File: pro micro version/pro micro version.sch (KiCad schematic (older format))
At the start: 78 parts, among them SW1 SW_PUSH, U1 ProMicro

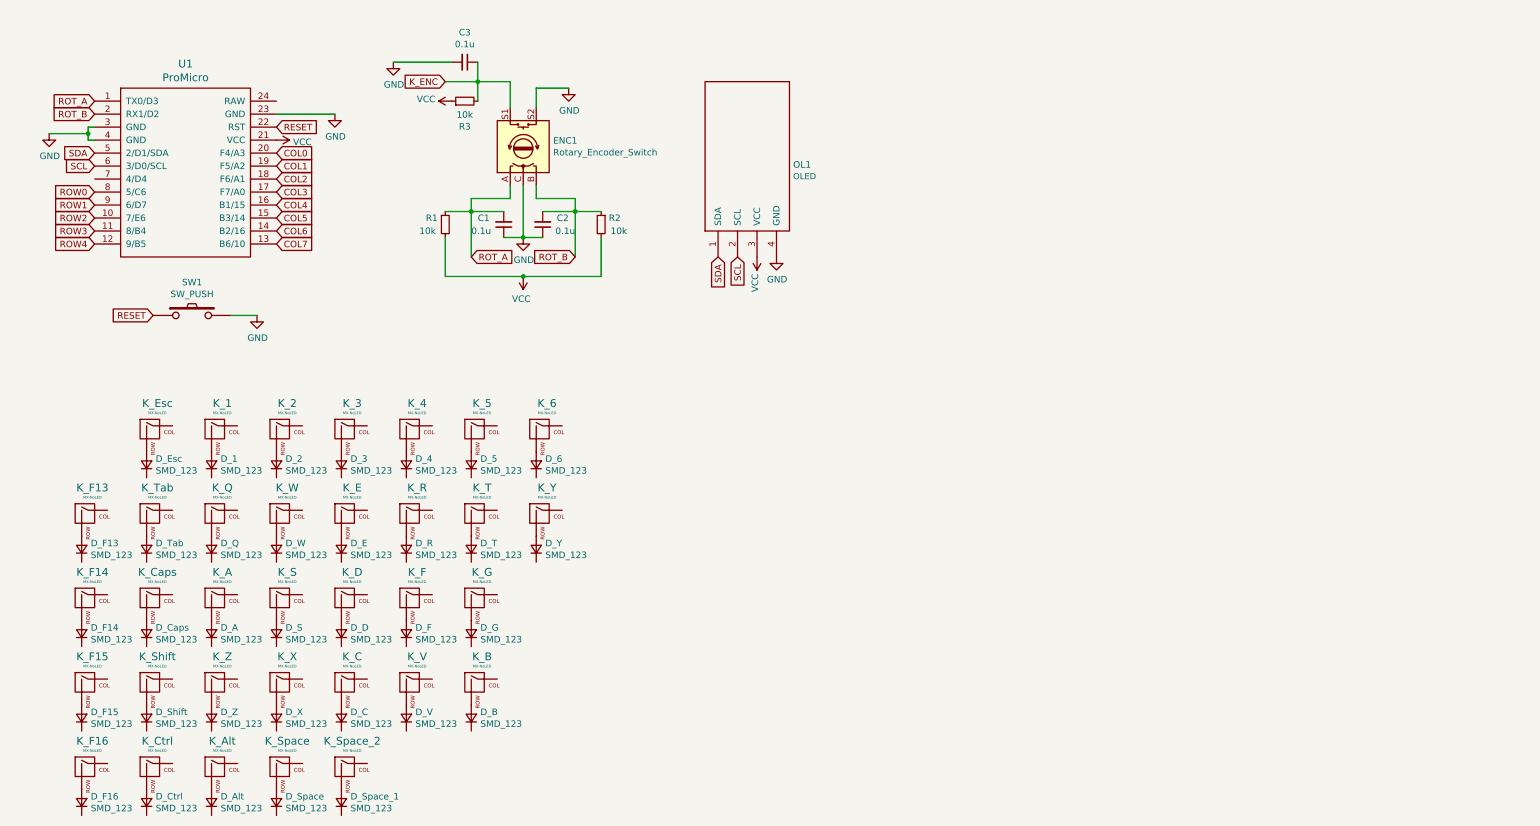
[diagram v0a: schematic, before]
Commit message: finished sechma
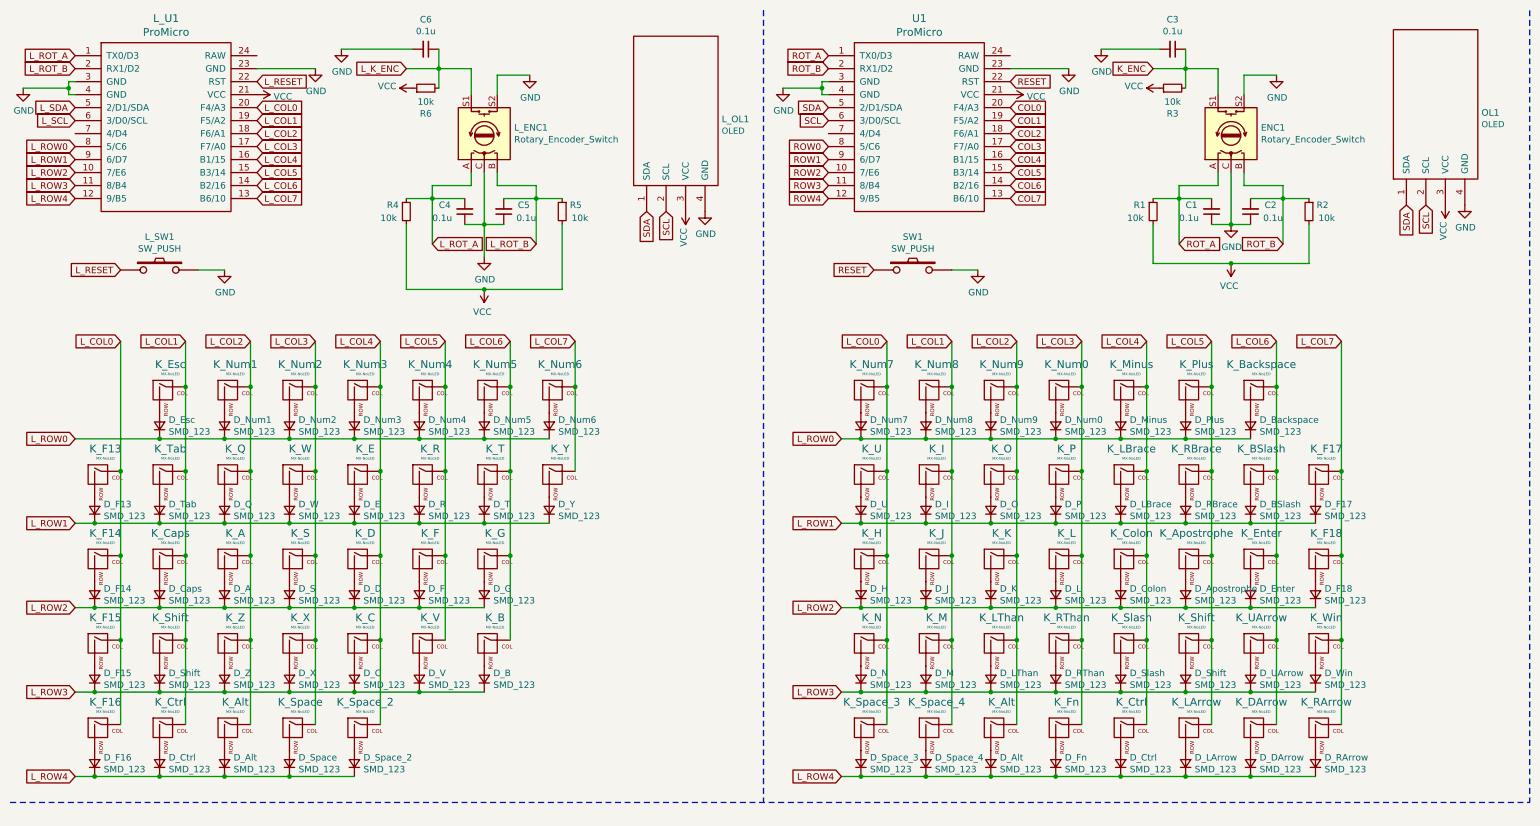
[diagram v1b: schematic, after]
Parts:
- added C1, C2, C3: 0.1u, symbol Device:C_Small
- added D_Alt, D_Apostrophe, D_BSlash, D_Backspace, D_Colon, D_Ctrl, D_DArrow, D_Enter, D_F17, D_F18, D_Fn, D_H, D_I, D_J, D_K, D_L, D_LArrow, D_LBrace, D_LThan, D_M, D_Minus, D_N, D_Num0, D_Num7, D_Num8, D_Num9, D_O, D_P, D_Plus, D_RArrow, D_RBrace, D_RThan, D_Shift, D_Slash, D_Space_3, D_Space_4, D_U, D_UArrow, D_Win: SMD_123, symbol Device:D_Small
- added ENC1: Rotary_Encoder_Switch, symbol Device:Rotary_Encoder_Switch
- added K_Alt, K_Apostrophe, K_BSlash, K_Backspace, K_Colon, K_Ctrl, K_DArrow, K_Enter, K_F17, K_F18, K_Fn, K_H, K_I, K_J, K_K, K_L, K_LArrow, K_LBrace, K_LThan, K_M, K_Minus, K_N, K_Num0, K_Num7, K_Num8, K_Num9, K_O, K_P, K_Plus, K_RArrow, K_RBrace, K_RThan, K_Shift, K_Slash, K_Space_3, K_Space_4, K_U, K_UArrow, K_Win: MX-NoLED, symbol MX_Alps_Hybrid:MX-NoLED
- added OL1: OLED, symbol kbd:OLED
- added R1, R2, R3: 10k, symbol Device:R_Small
- added SW1: SW_PUSH, symbol kbd:SW_PUSH
- added U1: ProMicro, symbol kbd:ProMicro
- renumbered C1 to C4, C2 to C5, C3 to C6, D_1 to D_Num1, D_2 to D_Num2, D_3 to D_Num3, D_4 to D_Num4, D_5 to D_Num5, D_6 to D_Num6, D_Space_1 to D_Space_2, K_1 to K_Num1, K_2 to K_Num2, K_3 to K_Num3, K_4 to K_Num4, K_5 to K_Num5, K_6 to K_Num6, ENC1 to L_ENC1, OL1 to L_OL1, SW1 to L_SW1, U1 to L_U1, R1 to R4, R2 to R5, R3 to R6
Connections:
- net COL0: now also U1.20 (F4/A3); no longer L_U1.20 (F4/A3)
- net COL1: now also U1.19 (F5/A2); no longer L_U1.19 (F5/A2)
- net COL2: now also U1.18 (F6/A1); no longer L_U1.18 (F6/A1)
- net COL3: now also U1.17 (F7/A0); no longer L_U1.17 (F7/A0)
- net COL4: now also U1.16 (B1/15); no longer L_U1.16 (B1/15)
- net COL5: now also U1.15 (B3/14); no longer L_U1.15 (B3/14)
- net COL6: now also U1.14 (B2/16); no longer L_U1.14 (B2/16)
- net COL7: now also U1.13 (B6/10); no longer L_U1.13 (B6/10)
- net GND: now also C1.1, C2.1, C3.2, ENC1.C, ENC1.S2, OL1.4 (GND), SW1.2, U1.23 (GND), U1.3 (GND), U1.4 (GND)
- net K_ENC: now also C3.1, ENC1.S1, R3.2; no longer C6.1, L_ENC1.S1, R6.2
- net RESET: now also SW1.1, U1.22 (RST); no longer L_SW1.1, L_U1.22 (RST)
- net ROT_A: now also C1.2, ENC1.A, R1.1, U1.1 (TX0/D3); no longer C4.2, L_ENC1.A, L_U1.1 (TX0/D3), R4.1
- net ROT_B: now also C2.2, ENC1.B, R2.1, U1.2 (RX1/D2); no longer C5.2, L_ENC1.B, L_U1.2 (RX1/D2), R5.1
- net ROW0: now also U1.8 (5/C6); no longer L_U1.8 (5/C6)
- net ROW1: now also U1.9 (6/D7); no longer L_U1.9 (6/D7)
- net ROW2: now also U1.10 (7/E6); no longer L_U1.10 (7/E6)
- net ROW3: now also U1.11 (8/B4); no longer L_U1.11 (8/B4)
- net ROW4: now also U1.12 (9/B5); no longer L_U1.12 (9/B5)
- net SCL: now also OL1.2 (SCL), U1.6 (3/D0/SCL); no longer L_U1.6 (3/D0/SCL)
- net SDA: now also OL1.1 (SDA), U1.5 (2/D1/SDA); no longer L_U1.5 (2/D1/SDA)
- net VCC: now also OL1.3 (VCC), R1.2, R2.2, R3.1, U1.21 (VCC)
- net L_COL1: now reaches K_Esc.1 (COL)
- net L_COL1: now also K_Caps.1 (COL), K_Ctrl.1 (COL), K_Shift.1 (COL), K_Tab.1 (COL), L_U1.19 (F5/A2), K_I.1 (COL), K_J.1 (COL), K_M.1 (COL), K_Num8.1 (COL), K_Space_4.1 (COL)
- net L_ROW0: now reaches D_Esc.1 (K)
- net L_ROW0: now also D_Num1.1 (K), D_Num2.1 (K), D_Num3.1 (K), D_Num4.1 (K), D_Num5.1 (K), D_Num6.1 (K), L_U1.8 (5/C6), D_Backspace.1 (K), D_Minus.1 (K), D_Num0.1 (K), D_Num7.1 (K), D_Num8.1 (K), D_Num9.1 (K), D_Plus.1 (K)
- net L_COL2: now reaches K_Num1.1 (COL)
- net L_COL2: now also K_A.1 (COL), K_Alt.1 (COL), K_Q.1 (COL), K_Z.1 (COL), L_U1.18 (F6/A1), K_Alt.1 (COL), K_K.1 (COL), K_LThan.1 (COL), K_Num9.1 (COL), K_O.1 (COL)
- net L_COL3: now reaches K_Num2.1 (COL)
- net L_COL3: now also K_S.1 (COL), K_Space.1 (COL), K_W.1 (COL), K_X.1 (COL), L_U1.17 (F7/A0), K_Fn.1 (COL), K_L.1 (COL), K_Num0.1 (COL), K_P.1 (COL), K_RThan.1 (COL)
- net L_COL4: now reaches K_Num3.1 (COL)
- net L_COL4: now also K_C.1 (COL), K_D.1 (COL), K_E.1 (COL), K_Space_2.1 (COL), L_U1.16 (B1/15), K_Colon.1 (COL), K_Ctrl.1 (COL), K_LBrace.1 (COL), K_Minus.1 (COL), K_Slash.1 (COL)
- net L_COL5: now reaches K_Num4.1 (COL)
- net L_COL5: now also K_F.1 (COL), K_R.1 (COL), K_V.1 (COL), L_U1.15 (B3/14), K_Apostrophe.1 (COL), K_LArrow.1 (COL), K_Plus.1 (COL), K_RBrace.1 (COL), K_Shift.1 (COL)
- net L_COL6: now reaches K_Num5.1 (COL)
- net L_COL6: now also K_B.1 (COL), K_G.1 (COL), K_T.1 (COL), L_U1.14 (B2/16), K_BSlash.1 (COL), K_Backspace.1 (COL), K_DArrow.1 (COL), K_Enter.1 (COL), K_UArrow.1 (COL)
- net L_COL7: now reaches K_Num6.1 (COL)
- net L_COL7: now also K_Y.1 (COL), L_U1.13 (B6/10), K_F17.1 (COL), K_F18.1 (COL), K_RArrow.1 (COL), K_Win.1 (COL)
- net L_COL0: now reaches K_F13.1 (COL)
- net L_COL0: now also K_F14.1 (COL), K_F15.1 (COL), K_F16.1 (COL), L_U1.20 (F4/A3), K_H.1 (COL), K_N.1 (COL), K_Num7.1 (COL), K_Space_3.1 (COL), K_U.1 (COL)
- net L_ROW1: now reaches D_Q.1 (K)
- net L_ROW1: now also D_E.1 (K), D_F13.1 (K), D_R.1 (K), D_T.1 (K), D_Tab.1 (K), D_W.1 (K), D_Y.1 (K), L_U1.9 (6/D7), D_BSlash.1 (K), D_F17.1 (K), D_I.1 (K), D_LBrace.1 (K), D_O.1 (K), D_P.1 (K), D_RBrace.1 (K), D_U.1 (K)
- net L_ROW2: now reaches D_Caps.1 (K)
- net L_ROW2: now also D_A.1 (K), D_D.1 (K), D_F.1 (K), D_F14.1 (K), D_G.1 (K), D_S.1 (K), L_U1.10 (7/E6), D_Apostrophe.1 (K), D_Colon.1 (K), D_Enter.1 (K), D_F18.1 (K), D_H.1 (K), D_J.1 (K), D_K.1 (K), D_L.1 (K)
- net L_ROW3: now reaches D_Shift.1 (K)
- net L_ROW3: now also D_B.1 (K), D_C.1 (K), D_F15.1 (K), D_V.1 (K), D_X.1 (K), D_Z.1 (K), L_U1.11 (8/B4), D_LThan.1 (K), D_M.1 (K), D_N.1 (K), D_RThan.1 (K), D_Shift.1 (K), D_Slash.1 (K), D_UArrow.1 (K), D_Win.1 (K)
- net L_ROW4: now reaches D_F16.1 (K)
- net L_ROW4: now also D_Alt.1 (K), D_Ctrl.1 (K), D_Space.1 (K), D_Space_2.1 (K), L_U1.12 (9/B5), D_Alt.1 (K), D_Ctrl.1 (K), D_DArrow.1 (K), D_Fn.1 (K), D_LArrow.1 (K), D_RArrow.1 (K), D_Space_3.1 (K), D_Space_4.1 (K)
- new net: D_Num7.2 (A), K_Num7.2 (ROW)
- new net: D_U.2 (A), K_U.2 (ROW)
- new net: D_H.2 (A), K_H.2 (ROW)
- new net: D_N.2 (A), K_N.2 (ROW)
- new net: D_Space_3.2 (A), K_Space_3.2 (ROW)
- new net: D_Num8.2 (A), K_Num8.2 (ROW)
- new net: D_I.2 (A), K_I.2 (ROW)
- new net: D_J.2 (A), K_J.2 (ROW)
- new net: D_M.2 (A), K_M.2 (ROW)
- new net: D_Space_4.2 (A), K_Space_4.2 (ROW)
- new net: D_Num9.2 (A), K_Num9.2 (ROW)
- new net: D_O.2 (A), K_O.2 (ROW)
- new net: D_K.2 (A), K_K.2 (ROW)
- new net: D_LThan.2 (A), K_LThan.2 (ROW)
- new net: D_Alt.2 (A), K_Alt.2 (ROW)
- new net: D_Num0.2 (A), K_Num0.2 (ROW)
- new net: D_P.2 (A), K_P.2 (ROW)
- new net: D_L.2 (A), K_L.2 (ROW)
- new net: D_RThan.2 (A), K_RThan.2 (ROW)
- new net: D_Fn.2 (A), K_Fn.2 (ROW)
- new net: D_Minus.2 (A), K_Minus.2 (ROW)
- new net: D_LBrace.2 (A), K_LBrace.2 (ROW)
- new net: D_Colon.2 (A), K_Colon.2 (ROW)
- new net: D_Slash.2 (A), K_Slash.2 (ROW)
- new net: D_Ctrl.2 (A), K_Ctrl.2 (ROW)
- new net: D_Plus.2 (A), K_Plus.2 (ROW)
- new net: D_RBrace.2 (A), K_RBrace.2 (ROW)
- new net: D_Apostrophe.2 (A), K_Apostrophe.2 (ROW)
- new net: D_Shift.2 (A), K_Shift.2 (ROW)
- new net: D_LArrow.2 (A), K_LArrow.2 (ROW)
- new net: D_Backspace.2 (A), K_Backspace.2 (ROW)
- new net: D_BSlash.2 (A), K_BSlash.2 (ROW)
- new net: D_Enter.2 (A), K_Enter.2 (ROW)
- new net: D_UArrow.2 (A), K_UArrow.2 (ROW)
- new net: D_DArrow.2 (A), K_DArrow.2 (ROW)
- new net: D_F17.2 (A), K_F17.2 (ROW)
- new net: D_F18.2 (A), K_F18.2 (ROW)
- new net: D_Win.2 (A), K_Win.2 (ROW)
- new net: D_RArrow.2 (A), K_RArrow.2 (ROW)
- new net L_K_ENC: C6.1, L_ENC1.S1, R6.2
- new net L_RESET: L_SW1.1, L_U1.22 (RST)
- new net L_ROT_A: C4.2, L_ENC1.A, L_U1.1 (TX0/D3), R4.1
- new net L_ROT_B: C5.2, L_ENC1.B, L_U1.2 (RX1/D2), R5.1
- new net L_SCL: L_U1.6 (3/D0/SCL)
- new net L_SDA: L_U1.5 (2/D1/SDA)
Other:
- moved on the sheet: C4, C5, C6, D_A, D_Alt, D_B, D_C, D_Caps, D_Ctrl, D_D, D_E, D_Esc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
